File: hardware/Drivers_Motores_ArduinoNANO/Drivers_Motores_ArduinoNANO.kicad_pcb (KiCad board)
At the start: 2 copper layers, 75 x 35 mm, 25 parts, among them J1 V+-, J2 FTDI, J3 RS485, P1 HEADER_02X05, P2 HEADER_02X05, U1 AMS1117-5.0, U2 ATMEGA328P-AU, Y1 16MHz

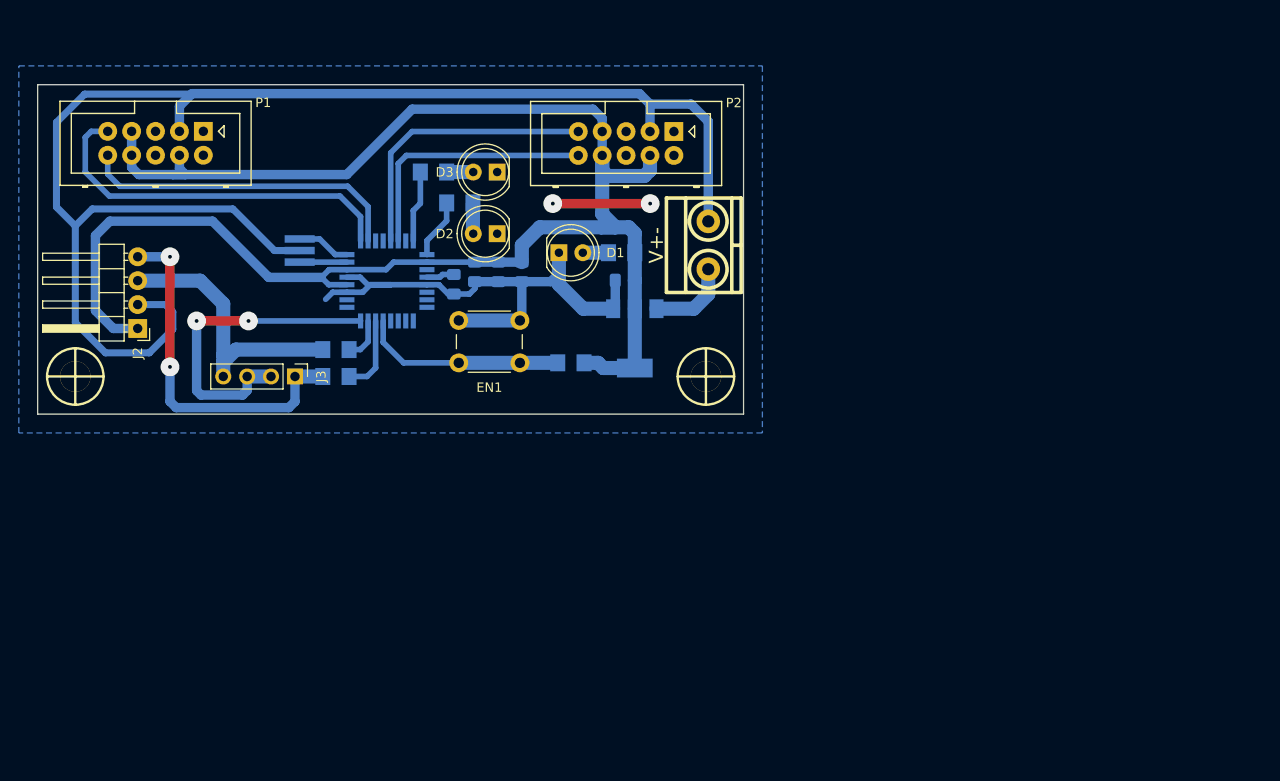
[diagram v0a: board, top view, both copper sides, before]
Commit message: Nuevo PCb
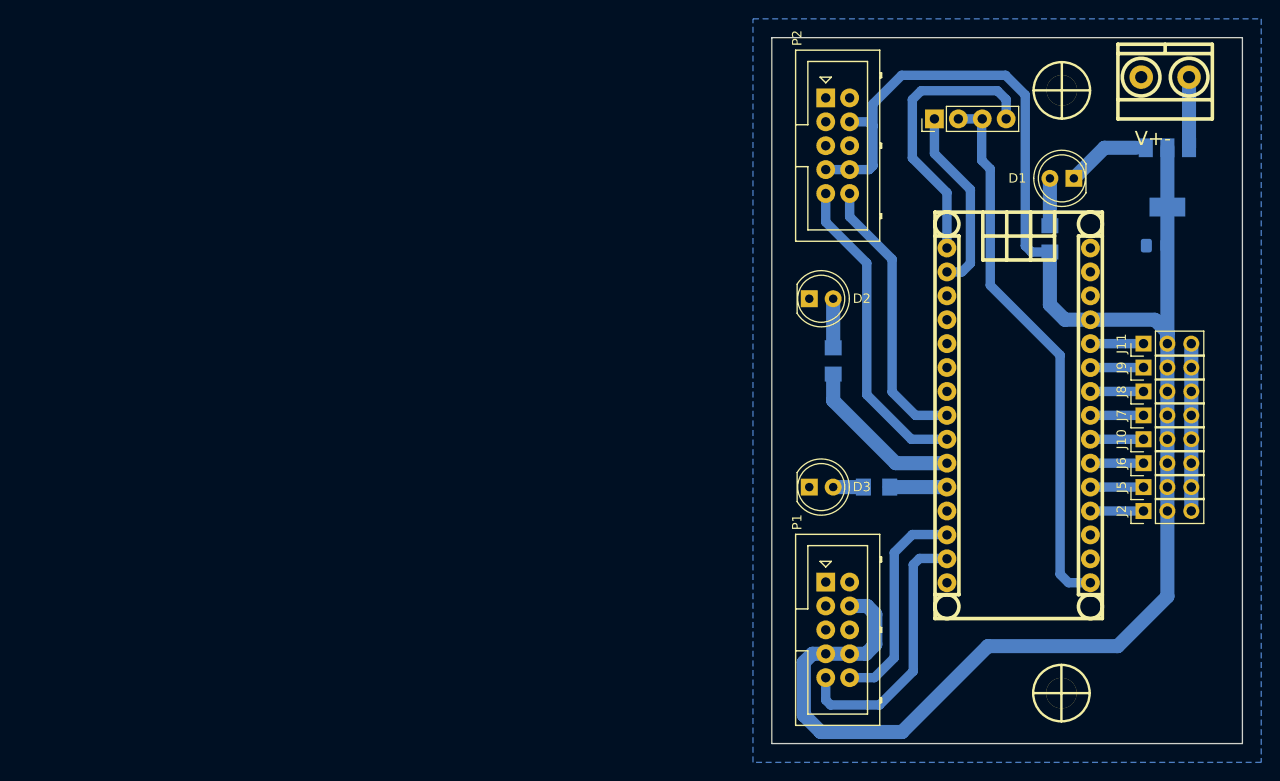
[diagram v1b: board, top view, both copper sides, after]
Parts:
- removed C2, C4: 1uF, Capacitor_SMD:C_0805_2012Metric_Pad1.18x1.45mm_HandSolder
- removed C3: 4,7uF, Capacitor_SMD:C_0805_2012Metric_Pad1.18x1.45mm_HandSolder
- removed C5: 100nF, Capacitor_SMD:C_0805_2012Metric_Pad1.18x1.45mm_HandSolder
- removed EN1: SW_Push, Button_Switch_THT:SW_PUSH_6mm_H5mm
- removed R1: 10K, EESTN5-v2:R_1206
- removed R3, R4: 1K, EESTN5-v2:R_1206
- removed U2: ATMEGA328P-AU, EESTN5-v2:TQFP-32_7x7mm_Pitch0.8mm
- removed Y1: 16MHz, Crystal:Resonator_SMD_Murata_CSTxExxV-3Pin_3.0x1.1mm_HandSoldering
- added J10: Conn, Connector_PinHeader_2.54mm:PinHeader_1x03_P2.54mm_Vertical, F.Cu at (218.5, 102.7)
- added J11: Conn, Connector_PinHeader_2.54mm:PinHeader_1x03_P2.54mm_Vertical, F.Cu at (218.5, 92.5)
- added J4: Arduino_Nano_Header, EESTN5-v2:arduino_nano_header, F.Cu at (205.2, 100.1)
- added J5: Conn, Connector_PinHeader_2.54mm:PinHeader_1x03_P2.54mm_Vertical, F.Cu at (218.5, 107.8)
- added J6: Conn, Connector_PinHeader_2.54mm:PinHeader_1x03_P2.54mm_Vertical, F.Cu at (218.5, 105.2)
- added J7: Conn, Connector_PinHeader_2.54mm:PinHeader_1x03_P2.54mm_Vertical, F.Cu at (218.5, 100.1)
- added J8: Conn, Connector_PinHeader_2.54mm:PinHeader_1x03_P2.54mm_Vertical, F.Cu at (218.5, 97.6)
- added J9: Conn, Connector_PinHeader_2.54mm:PinHeader_1x03_P2.54mm_Vertical, F.Cu at (218.5, 95.0)
- J2: value FTDI -> Conn; footprint Connector_PinHeader_2.54mm:PinHeader_1x04_P2.54mm_Horizontal -> Connector_PinHeader_2.54mm:PinHeader_1x03_P2.54mm_Vertical
- moved H1 110.0 mm to (209.8, 129.6), turned to 90 degrees
- moved J2 108.6 mm to (218.5, 110.3), turned to 90 degrees
- moved P1 89.0 mm to (186.0, 122.9), turned to -90 degrees
- moved J3 73.2 mm to (196.3, 68.6), turned to 90 degrees
- moved U1 59.1 mm to (221.0, 74.8)
- moved R6 57.8 mm to (190.1, 107.8), turned to 0 degrees
- moved C1 56.5 mm to (219.8, 82.1)
- moved D1 55.3 mm to (211.1, 75.0), turned to 180 degrees
- moved J1 51.7 mm to (220.8, 64.2), turned to 180 degrees
- moved H2 48.5 mm to (209.8, 65.6), turned to 90 degrees
- moved D3 47.1 mm to (183.0, 107.8), turned to 0 degrees
- moved R2 45.5 mm to (208.5, 81.4), turned to 90 degrees
- moved R5 43.1 mm to (185.5, 94.3), turned to -90 degrees
- moved D2 33.9 mm to (183.0, 87.7), turned to 0 degrees
- moved P2 22.5 mm to (186.0, 71.5), turned to -90 degrees
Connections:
- J2 pad 1: +5V -> /1
- J2 pad 2: GND -> +5V
- J2 pad 3: /Tx -> GND
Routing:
- net GND: track 225.7 -> 25.7 mm, vias 2 -> 0
- net /DERE: track 34.6 -> 58.0 mm, vias 2 -> 0
- net /RESET: track 21.7 -> 0.00 mm
- net /Rx: track 38.2 -> 19.8 mm, vias 2 -> 0
- net /M1B: track 40.1 -> 28.6 mm
- net /M1A: track 34.7 -> 23.2 mm
- net /LED_2: track 6.36 -> 17.7 mm
- net /D0/RX: track 8.19 -> 0.00 mm
- net Net-(U2-(PCINT7/XTAL2/TOSC2)PB7): track 5.71 -> 0.00 mm
- net /8: track 0.00 -> 5.64 mm
- net /7: track 0.00 -> 5.64 mm
- net /6: track 0.00 -> 5.64 mm
- net /5: track 0.00 -> 5.64 mm
- net /4: track 0.00 -> 5.64 mm
- net /3: track 0.00 -> 5.64 mm
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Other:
- board size 75 x 35 mm -> 50 x 75 mm
